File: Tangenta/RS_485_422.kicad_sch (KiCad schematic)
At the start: 40 parts, among them J15 Conn_01x06_Pin, Q3 BSS138, U21 TPCDSOT23-SM712, U22 TPCDSOT23-SM712

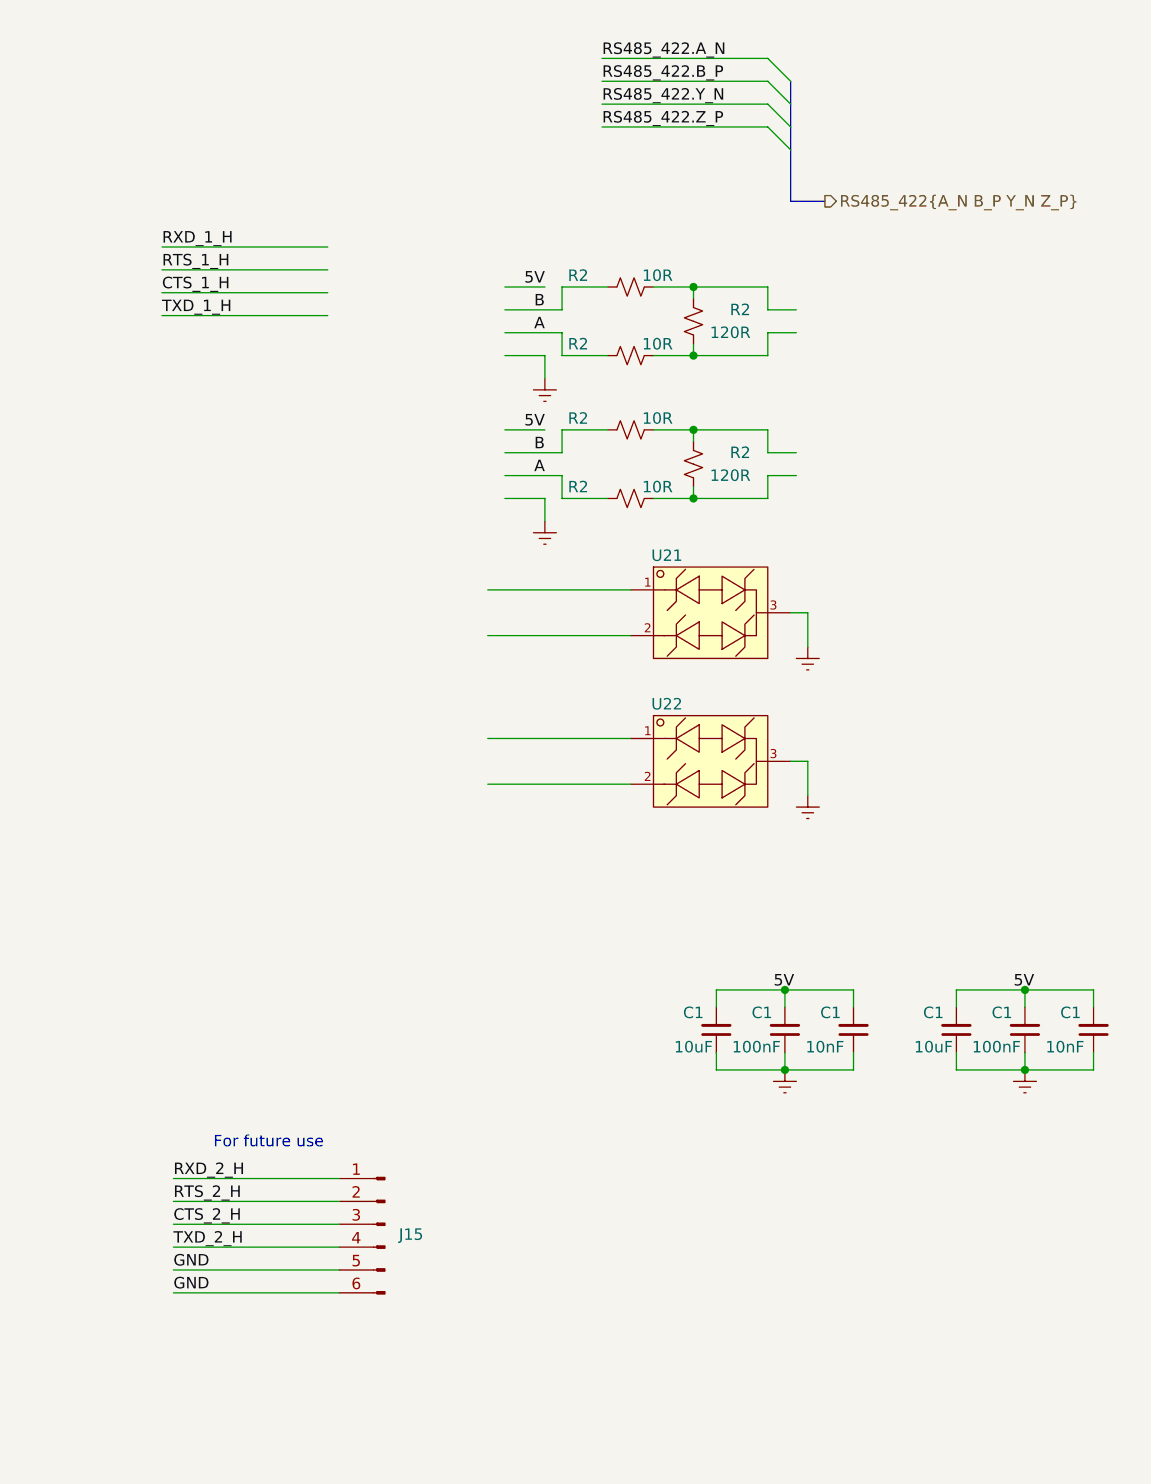
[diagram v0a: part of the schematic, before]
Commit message: ...
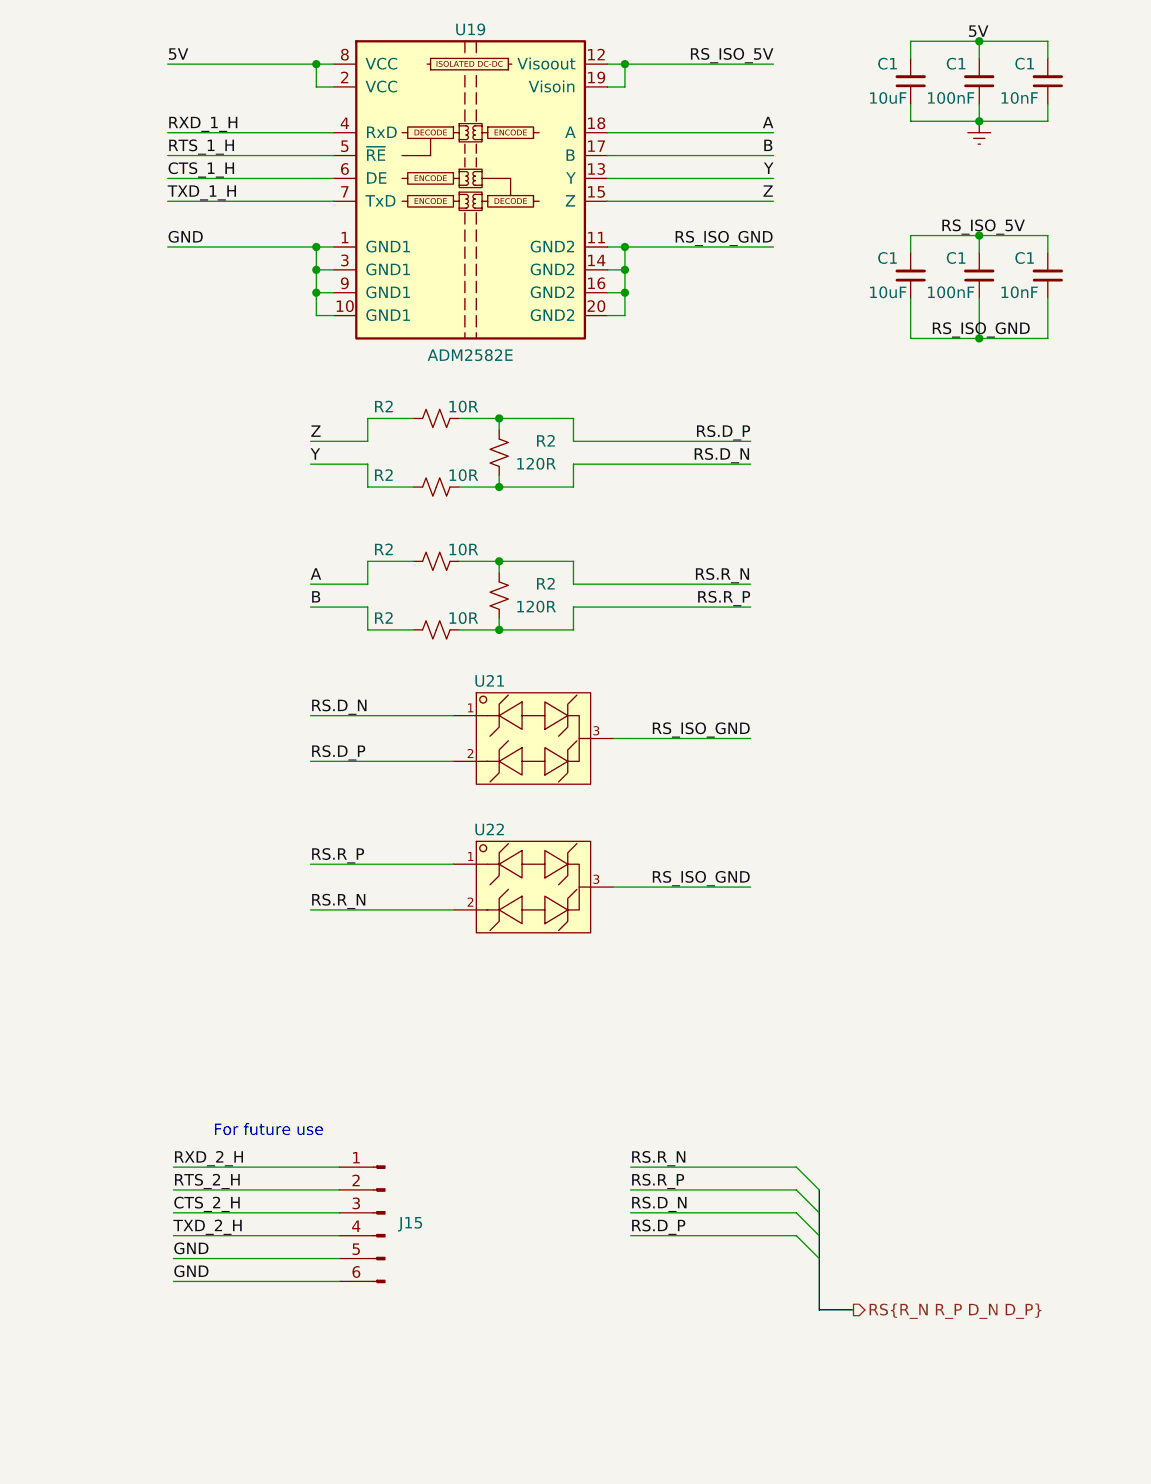
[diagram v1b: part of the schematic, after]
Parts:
- added U19: ADM2582E, Package_SO:SOIC-20W_7.5x12.8mm_P1.27mm, symbol Interface_UART:ADM2582E
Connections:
- net 5V: now also U19.2 (VCC), U19.8 (VCC); no longer C1.2, C1.2, C1.2
- net A: now also R2.2, U19.18 (A); no longer R2.2, R2.2
- net B: now also R2.2, U19.17 (B); no longer R2.2, R2.2
- net CTS_1_H: now also U19.6 (DE)
- net GNDREF: now also U19.1 (GND1), U19.10 (GND1), U19.3 (GND1), U19.9 (GND1); no longer C1.1, C1.1, C1.1, U21.3, U22.3
- net RTS_1_H: now also U19.5 (~{RE})
- net RXD_1_H: now also U19.4 (RxD)
- net TXD_1_H: now also U19.7 (TxD)
- net RS.R_P: now reaches R2.1, R2.1
- net RS.R_P: now also U22.1
- net RS.R_N: now reaches R2.1, R2.2
- net RS.R_N: now also U22.2
- net RS.D_P: now reaches R2.1, R2.2
- net RS.D_P: now also U21.2
- net RS.D_N: now reaches R2.1, R2.1
- net RS.D_N: now also U21.1
- new net RS_ISO_5V: C1.2, C1.2, C1.2, U19.12 (Visoout), U19.19 (Visoin)
- new net RS_ISO_GND: C1.1, C1.1, C1.1, U19.11 (GND2), U19.14 (GND2), U19.16 (GND2), U19.20 (GND2), U21.3, U22.3
- new net Y: R2.2, U19.13 (Y)
- new net Z: R2.2, U19.15 (Z)
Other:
- moved on the sheet: C1, J15, R2, U21, U22
